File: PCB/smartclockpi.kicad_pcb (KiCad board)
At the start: 2 copper layers, 17 parts, among them J1 Raspberry_Pi_2_3, J2 DS3231 RTC module, J3 ILI9488 SPI TFT touchscreen, J4 PCM5102A DAC (with headphone 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, U1 BME280, U2 MCP3008

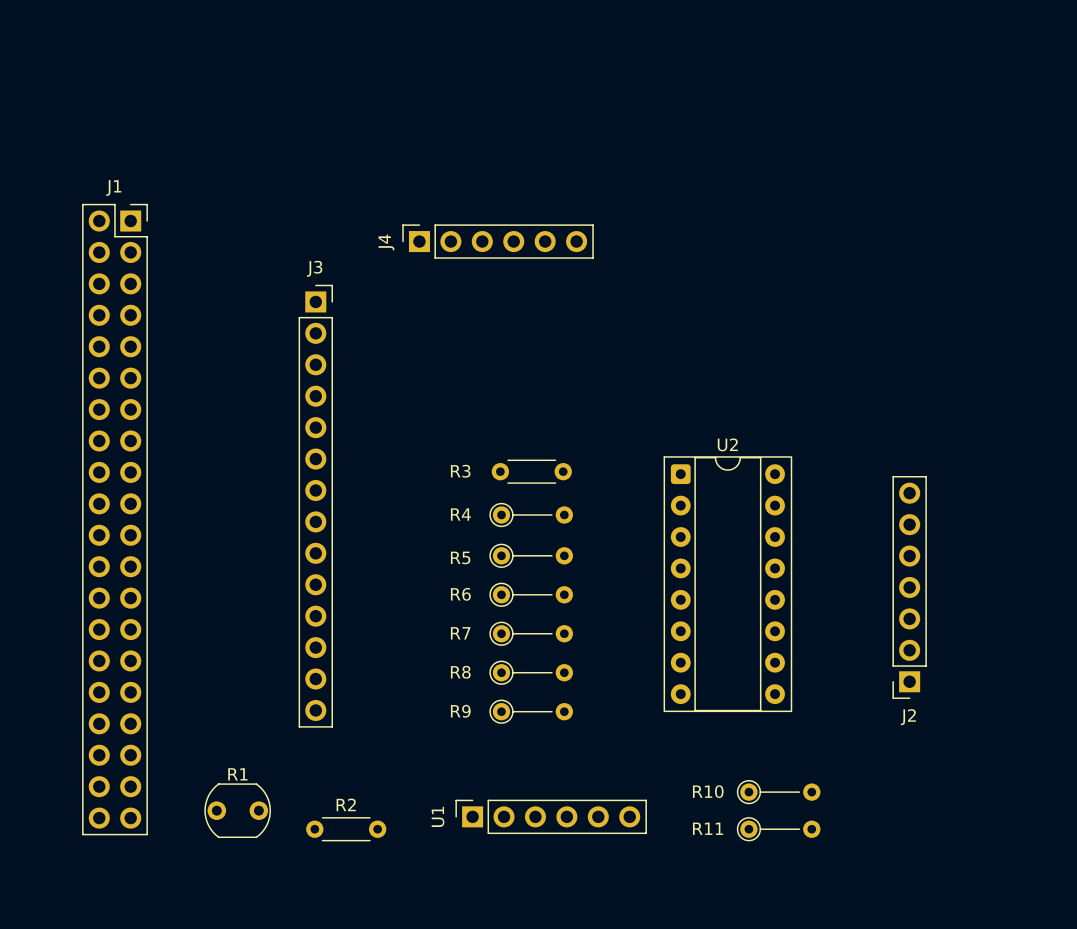
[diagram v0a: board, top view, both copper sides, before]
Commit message: finallise pcb. spent toooo much time on this...
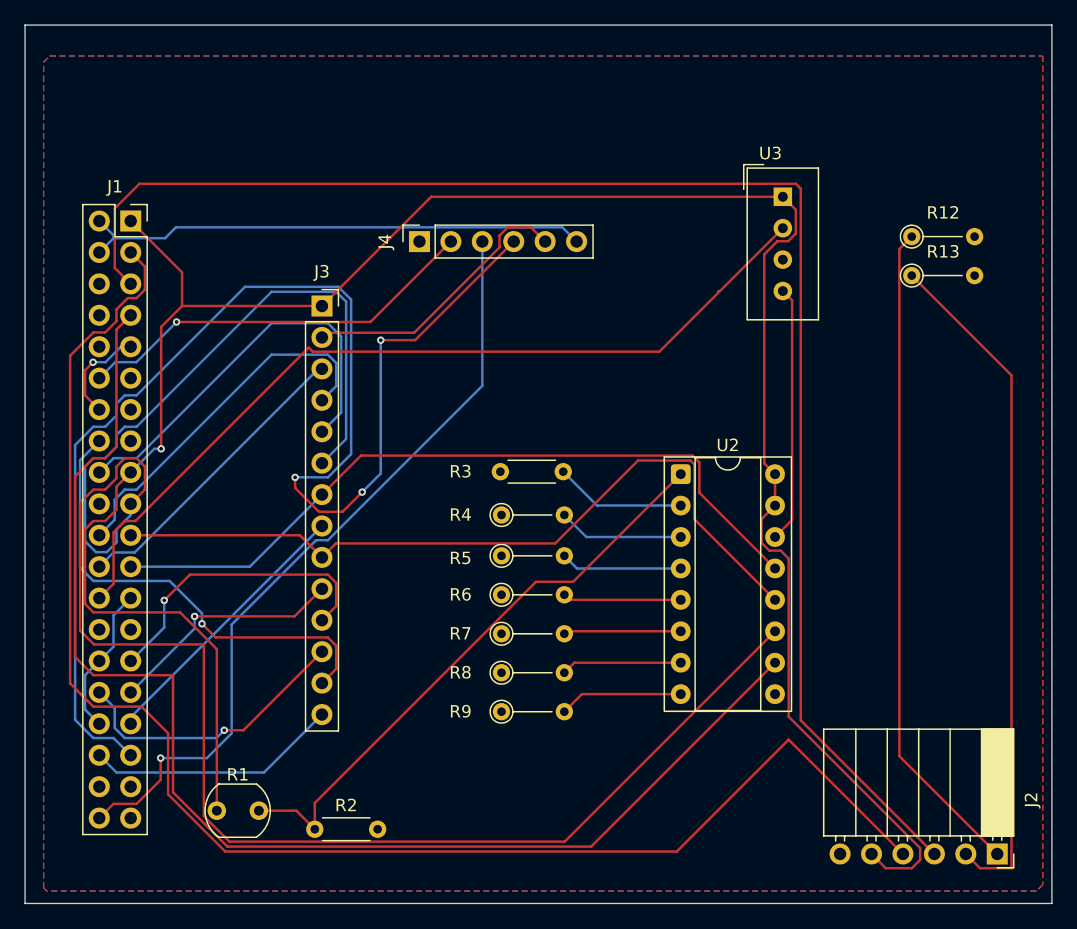
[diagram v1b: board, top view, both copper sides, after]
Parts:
- removed R10, R11: 4.7kΩ, Resistor_THT:R_Axial_DIN0204_L3.6mm_D1.6mm_P5.08mm_Vertical
- removed U1: BME280, Connector_PinSocket_2.54mm:PinSocket_1x06_P2.54mm_Vertical
- added R12: 4.7kΩ, Resistor_THT:R_Axial_DIN0204_L3.6mm_D1.6mm_P5.08mm_Vertical, F.Cu at (110.2, 83.1)
- added R13: 4.7kΩ, Resistor_THT:R_Axial_DIN0204_L3.6mm_D1.6mm_P5.08mm_Vertical, F.Cu at (110.2, 86.2)
- added U3: DHT22, Sensor:Aosong_DHT11_5.5x12.0_P2.54mm, F.Cu at (99.8, 79.9)
- J2: footprint Connector_PinSocket_2.54mm:PinSocket_1x07_P2.54mm_Vertical -> Connector_PinSocket_2.54mm:PinSocket_1x06_P2.54mm_Horizontal
- moved J2 15.6 mm to (117.1, 133.0), turned to -90 degrees
- moved J3 0.60 mm to (62.5, 88.7)
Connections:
- J1 pad 26: unconnected-(J1-~{CE1}/GPIO7-Pad26) -> Net-(J1-~{CE1}/GPIO7)
- J2 pad 1: (no net) -> Net-(J2-32K)
- J2 pad 2: (no net) -> Net-(J2-SQW)
- J2 pad 3: (no net) -> Net-(J1-SCL/GPIO3)
- J2 pad 4: (no net) -> Net-(J1-SDA/GPIO2)
- J2 pad 5: (no net) -> +3.3V
- J2 pad 6: (no net) -> GND
- J3 pad 1: (no net) -> +3.3V
- J3 pad 10: (no net) -> Net-(J1-GCLK2/GPIO6)
- J3 pad 11: (no net) -> Net-(J1-GCLK1/GPIO5)
- J3 pad 12: (no net) -> Net-(J1-PWM0/GPIO12)
- J3 pad 13: (no net) -> Net-(J1-GPIO23)
- J3 pad 14: (no net) -> Net-(J1-GPIO16)
- J3 pad 2: (no net) -> GND
- J3 pad 3: (no net) -> Net-(J1-~{CE0}/GPIO8)
- J3 pad 4: (no net) -> Net-(J1-GPIO25)
- J3 pad 5: (no net) -> Net-(J1-GPIO24)
- J3 pad 6: (no net) -> Net-(J1-MOSI0/GPIO10)
- J3 pad 7: (no net) -> Net-(J1-SCLK0/GPIO11)
- J3 pad 8: (no net) -> Net-(J1-PWM1/GPIO13)
- J3 pad 9: (no net) -> Net-(J1-MISO0/GPIO9)
- J4 pad 1: (no net) -> unconnected-(J4-SCK-Pad1)
- J4 pad 2: (no net) -> Net-(J1-GPIO18/PWM0)
- J4 pad 3: (no net) -> Net-(J1-GPIO21/SCLK1)
- J4 pad 4: (no net) -> Net-(J1-GPIO19/MISO1)
- J4 pad 5: (no net) -> GND
- J4 pad 6: (no net) -> +5V
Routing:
- net +3.3V: track 0.00 -> 181.2 mm, vias 0 -> 1
- net Net-(J1-MOSI0/GPIO10): track 0.00 -> 154.4 mm
- net Net-(J1-SDA/GPIO2): track 0.00 -> 122.2 mm
- net Net-(J1-SCL/GPIO3): track 0.00 -> 121.3 mm
- net Net-(J1-GPIO19/MISO1): track 0.00 -> 108.9 mm, vias 0 -> 3
- net Net-(J1-GCLK0/GPIO4): track 0.00 -> 104.7 mm
- net Net-(J1-~{CE1}/GPIO7): track 0.00 -> 70.3 mm
- net GND: track 0.00 -> 63.9 mm, vias 0 -> 1
- net Net-(J1-MISO0/GPIO9): track 0.00 -> 63.8 mm
- net Net-(J1-GPIO21/SCLK1): track 0.00 -> 63.3 mm, vias 0 -> 1
- net Net-(J1-SCLK0/GPIO11): track 0.00 -> 61.0 mm
- net Net-(J2-SQW): track 0.00 -> 55.4 mm
- net Net-(J2-32K): track 0.00 -> 53.6 mm
- net Net-(U2-CH0): track 0.00 -> 47.9 mm
- net +5V: track 0.00 -> 41.8 mm
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- added copper zone on B.Cu, net GND
- added copper zone on F.Cu, net GND
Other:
- board outline added: 83 x 71 mm
